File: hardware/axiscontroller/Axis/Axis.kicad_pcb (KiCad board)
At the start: 4 copper layers, 90 x 55 mm, 63 parts, among them J1 RS485, J10 Fan, J2 Motor, J3 Limits, J4 RS485, J5 Console, J6 Temp A, J7 Temp B, J8 Brake, J9 Power, Q4 IRLR8726TRPBF, Q5 IRLR8726TRPBF, SW1 SW_DIP_x04, U4 TLP291, U5 TLP291, U6 TLP291, U7 MAX485CPA, U8 74AHCT125

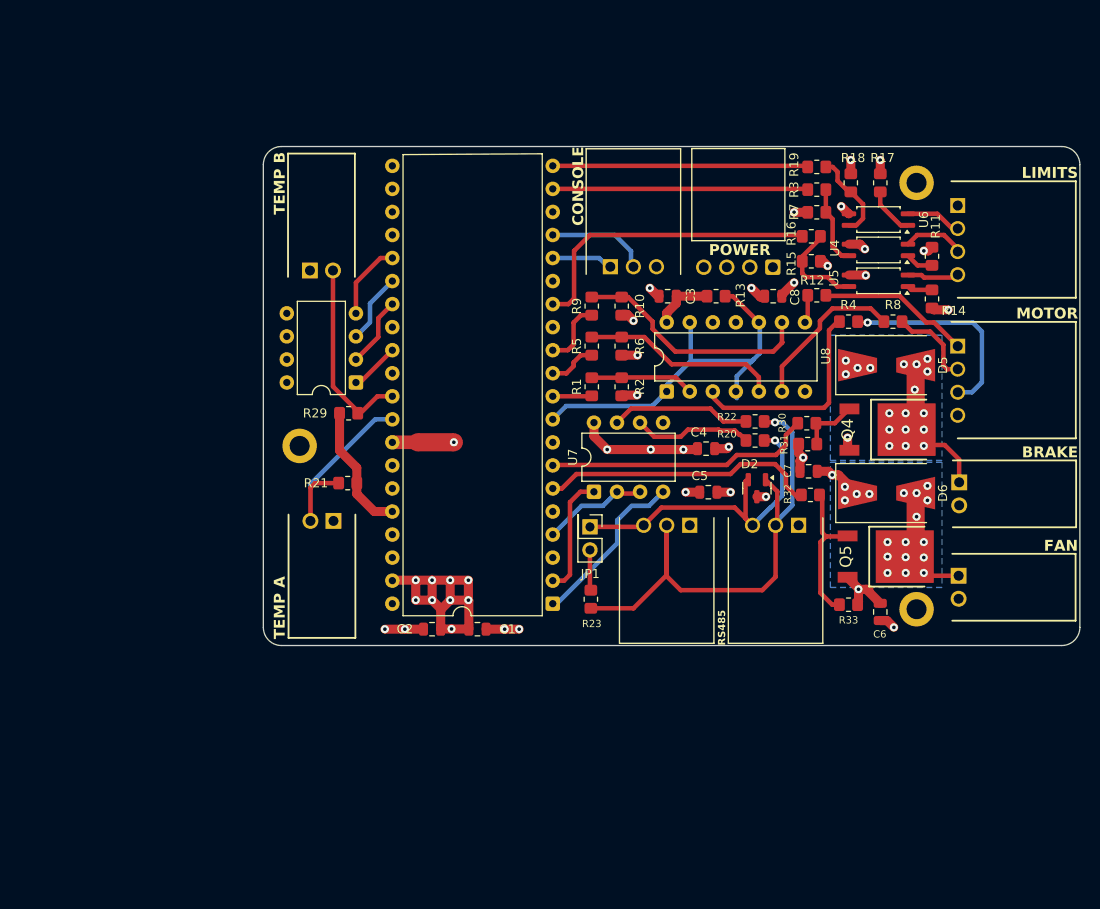
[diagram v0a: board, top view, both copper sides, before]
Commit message: The second revision of the robot axis controller.
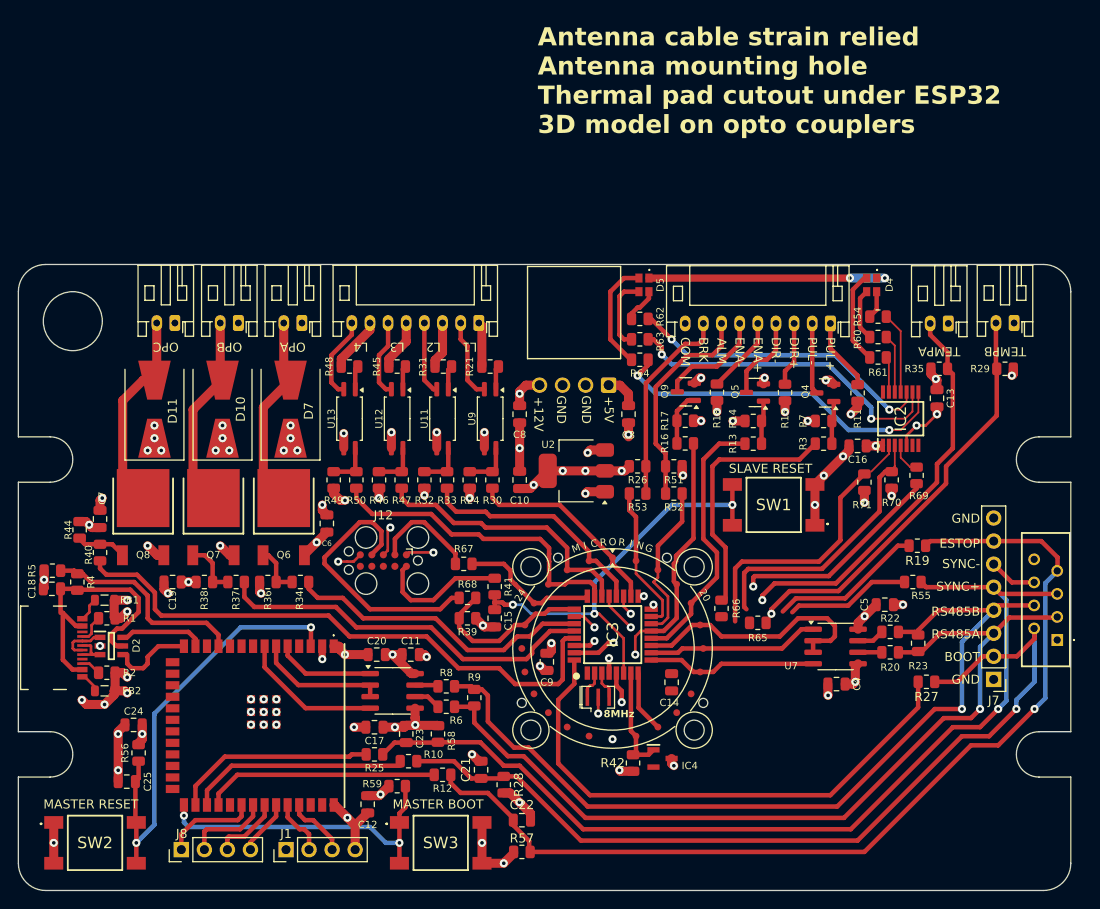
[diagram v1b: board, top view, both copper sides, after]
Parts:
- removed A1: RaspberryPi_Pico_W, AJS_Roberta:PI_PICO2_SOCKET
- removed C1: 100nF, Capacitor_SMD:C_0805_2012Metric
- removed C2: 47uF, Capacitor_SMD:C_0805_2012Metric
- removed D6: Schottky, Diode_SMD:D_SMB-SMC_Universal_Handsoldering
- removed H2, H3: MountingHole_Pad, MountingHole:MountingHole_2.2mm_M2_DIN965_Pad
- removed J10: Fan, AJS_Roberta:MOLEX_SL_70553_0001
- removed J9: Power, AJS_Roberta:MOLEX-171857-0001
- removed JP1: Termination, Connector_PinHeader_2.54mm:PinHeader_2x01_P2.54mm_Vertical
- removed NT1: NetTie_2, NetTie:NetTie-2_SMD_Pad2.0mm
- removed U4, U5, U6: TLP291, Package_SO:SOIC-4_4.55x2.6mm_P1.27mm
- removed U8: 74AHCT125, Package_DIP:DIP-14_W7.62mm
- added C10: 10uF, Capacitor_SMD:C_0805_2012Metric, F.Cu at (210.2, 103.8)
- added C11: 47uF, Capacitor_SMD:C_0805_2012Metric, F.Cu at (198.2, 123.0)
- added C12: 22uF, Capacitor_SMD:C_0805_2012Metric, F.Cu at (193.5, 139.5)
- added C13: 47uF, Capacitor_SMD:C_0805_2012Metric, F.Cu at (256.2, 94.8)
- added C14: 4.7uF, Capacitor_SMD:C_0805_2012Metric, F.Cu at (227.0, 126.0)
- added C15: 100nF, Capacitor_SMD:C_0805_2012Metric, F.Cu at (207.5, 119.0)
- added C16: 100nF, Capacitor_SMD:C_0805_2012Metric, F.Cu at (247.5, 100.0)
- added C17: 100nF, Capacitor_SMD:C_0805_2012Metric, F.Cu at (194.2, 131.0)
- added C18: 100nF, Capacitor_SMD:C_0805_2012Metric, F.Cu at (158.7, 115.8)
- added C19: 100nF, Capacitor_SMD:C_0805_2012Metric, F.Cu at (172.0, 115.0)
- added C20: 100nF, Capacitor_SMD:C_0805_2012Metric, F.Cu at (194.5, 123.0)
- added C21: 22nF, Capacitor_SMD:C_0805_2012Metric, F.Cu at (206.0, 135.7)
- added C22: 22nF, Capacitor_SMD:C_0805_2012Metric, F.Cu at (210.5, 141.2)
- added C23: 22nF, Capacitor_SMD:C_0805_2012Metric, F.Cu at (197.8, 131.8)
- added C24: 22uF, Capacitor_SMD:C_0805_2012Metric, F.Cu at (167.7, 130.8)
- added C25: 1uF, Capacitor_SMD:C_0805_2012Metric, F.Cu at (166.9, 137.0)
- added C9: 100nF, Capacitor_SMD:C_0805_2012Metric, F.Cu at (213.2, 123.8)
- added D10: Schottky, Diode_SMD:D_SMB-SMC_Universal_Handsoldering, F.Cu at (177.5, 96.0)
- added D11: Schottky, Diode_SMD:D_SMB-SMC_Universal_Handsoldering, F.Cu at (170.0, 96.0)
- added D4: CLMUD_FKC, AJS_Cree:CLMVC-FKC-CG1J1561BB7D3S3, F.Cu at (249.1, 82.2)
- added D7: Schottky, Diode_SMD:D_SMB-SMC_Universal_Handsoldering, F.Cu at (185.0, 96.0)
- added FB1: FerriteBead_Small, Inductor_SMD:L_0805_2012Metric, F.Cu at (164.5, 117.0)
- added FB2: FerriteBead_Small, Inductor_SMD:L_0805_2012Metric, F.Cu at (164.5, 127.0)
- added IC1: ESP32-S3-WROOM-1U-N16R8, AJS_Espressif:ESP32-S-3WROOM-1U-N16R8, F.Cu at (181.3, 130.8)
- added IC2: TCA6507PWR, AJS_TexasInstruments:TCA6507PWR, F.Cu at (252.2, 97.0)
- added IC3: STM32G071KBT3TR, AJS_STMicro:STM32G071KBT3TR, F.Cu at (220.5, 120.8)
- added IC4: AT21CS01-STUM10-T, AJS_STMicro:AT21CS01-STUM10-T, F.Cu at (226.0, 134.4)
- added J12: TC2050, Connector:Tag-Connect_TC2050-IDC-FP_2x05_P1.27mm_Vertical, F.Cu at (195.2, 112.6)
- added J17: JST PH, Connector_JST:JST_PH_S2B-PH-K_1x02_P2.00mm_Horizontal, F.Cu at (179.2, 86.5)
- added J18: JST PH, Connector_JST:JST_PH_S8B-PH-K_1x08_P2.00mm_Horizontal, F.Cu at (205.8, 86.5)
- added J19: JST PH, Connector_JST:JST_PH_S2B-PH-K_1x02_P2.00mm_Horizontal, F.Cu at (186.2, 86.5)
- added J20: JST PH, Connector_JST:JST_PH_S2B-PH-K_1x02_P2.00mm_Horizontal, F.Cu at (172.2, 86.5)
- added J21: JST PH, Connector_JST:JST_PH_S2B-PH-K_1x02_P2.00mm_Horizontal, F.Cu at (257.5, 86.5)
- added J22: JST PH, Connector_JST:JST_PH_S2B-PH-K_1x02_P2.00mm_Horizontal, F.Cu at (264.8, 86.5)
- added Q6: IRLR8726TRPBF, AJS_Roberta:IRLR8726TRPBF, F.Cu at (184.2, 107.8)
- added Q7: IRLR8726TRPBF, AJS_Roberta:IRLR8726TRPBF, F.Cu at (176.5, 107.8)
- added Q8: IRLR8726TRPBF, AJS_Roberta:IRLR8726TRPBF, F.Cu at (168.8, 107.8)
- added Q9: 2N7002, Package_TO_SOT_SMD:SOT-23, F.Cu at (228.6, 94.0)
- added R24: 4700, Resistor_SMD:R_0805_2012Metric, F.Cu at (204.8, 103.8)
- added R25: 33, Resistor_SMD:R_0805_2012Metric, F.Cu at (194.2, 134.0)
- added R26: 100K, Resistor_SMD:R_0805_2012Metric, F.Cu at (223.2, 102.2)
- added R27: 100, Resistor_SMD:R_0805_2012Metric, F.Cu at (255.1, 126.0)
- added R28: 4K7, Resistor_SMD:R_0805_2012Metric, F.Cu at (208.5, 137.3)
- added R34: 100, Resistor_SMD:R_0805_2012Metric, F.Cu at (186.1, 115.0)
- added R35: 10000, Resistor_SMD:R_0805_2012Metric, F.Cu at (256.5, 91.5)
- added R36: 10000, Resistor_SMD:R_0805_2012Metric, F.Cu at (182.5, 115.0)
- added R37: 100, Resistor_SMD:R_0805_2012Metric, F.Cu at (179.0, 115.0)
- added R38: 10000, Resistor_SMD:R_0805_2012Metric, F.Cu at (175.5, 115.0)
- added R39: 100K, Resistor_SMD:R_0805_2012Metric, F.Cu at (204.5, 119.0)
- added R40: 100, Resistor_SMD:R_0805_2012Metric, F.Cu at (164.0, 111.8)
- added R41: 100, Resistor_SMD:R_0805_2012Metric, F.Cu at (207.5, 115.5)
- added R42: 1K0, Resistor_SMD:R_0805_2012Metric, F.Cu at (222.8, 134.9)
- added R44: 10000, Resistor_SMD:R_0805_2012Metric, F.Cu at (161.8, 109.2)
- added R45: 1000, Resistor_SMD:R_0805_2012Metric, F.Cu at (196.8, 91.2)
- added R46: 4700, Resistor_SMD:R_0805_2012Metric, F.Cu at (194.8, 103.8)
- added R47: 100, Resistor_SMD:R_0805_2012Metric, F.Cu at (197.2, 103.8)
- added R48: 1000, Resistor_SMD:R_0805_2012Metric, F.Cu at (191.5, 91.2)
- added R49: 4700, Resistor_SMD:R_0805_2012Metric, F.Cu at (189.8, 103.8)
- added R50: 100, Resistor_SMD:R_0805_2012Metric, F.Cu at (192.2, 103.8)
- added R51: 100K, Resistor_SMD:R_0805_2012Metric, F.Cu at (227.2, 102.2)
- added R52: 100, Resistor_SMD:R_0805_2012Metric, F.Cu at (227.2, 105.2)
- added R53: 100, Resistor_SMD:R_0805_2012Metric, F.Cu at (223.2, 105.2)
- added R54: 330, Resistor_SMD:R_0805_2012Metric, F.Cu at (249.8, 85.8)
- added R55: 100, Resistor_SMD:R_0805_2012Metric, F.Cu at (253.6, 115.0)
- added R56: R_10K, Resistor_SMD:R_0805_2012Metric, F.Cu at (168.2, 133.8)
- added R57: 4K7, Resistor_SMD:R_0805_2012Metric, F.Cu at (210.5, 144.8)
- added R58: 4K7, Resistor_SMD:R_0805_2012Metric, F.Cu at (201.2, 131.8)
- added R59: R_10K, Resistor_SMD:R_0805_2012Metric, F.Cu at (196.8, 137.5)
- added R60: 330, Resistor_SMD:R_0805_2012Metric, F.Cu at (249.8, 88.0)
- added R61: 330, Resistor_SMD:R_0805_2012Metric, F.Cu at (249.8, 90.2)
- added R62: 330, Resistor_SMD:R_0805_2012Metric, F.Cu at (223.5, 86.0)
- added R63: 330, Resistor_SMD:R_0805_2012Metric, F.Cu at (223.5, 88.2)
- added R64: 330, Resistor_SMD:R_0805_2012Metric, F.Cu at (223.5, 90.5)
- added R65: 33, Resistor_SMD:R_0805_2012Metric, F.Cu at (236.5, 119.5)
- added R66: 33, Resistor_SMD:R_0805_2012Metric, F.Cu at (232.5, 117.9)
- added R67: 33, Resistor_SMD:R_0805_2012Metric, F.Cu at (204.1, 113.0)
- added R68: 33, Resistor_SMD:R_0805_2012Metric, F.Cu at (204.5, 116.8)
- added R69: 33, Resistor_SMD:R_0805_2012Metric, F.Cu at (254.0, 103.2)
- added R70: 4K7, Resistor_SMD:R_0805_2012Metric, F.Cu at (251.2, 103.8)
- added R71: 4K7, Resistor_SMD:R_0805_2012Metric, F.Cu at (248.2, 104.0)
- added SW2: SW_Tactile_6mm, AJS_SameSky:Tactile_6mm_6mm_4.5mm, F.Cu at (163.4, 143.8)
- added SW3: SW_Tactile_6mm, AJS_SameSky:Tactile_6mm_6mm_4.5mm, F.Cu at (201.6, 143.8)
- added U11: TLP291, Package_SO:SOIC-4_4.55x2.6mm_P1.27mm, F.Cu at (201.8, 97.0)
- added U12: TLP291, Package_SO:SOIC-4_4.55x2.6mm_P1.27mm, F.Cu at (196.8, 97.0)
- added U13: TLP291, Package_SO:SOIC-4_4.55x2.6mm_P1.27mm, F.Cu at (191.5, 97.0)
- added U14: MAX485CPA, Package_SO:SOIC-8_3.9x4.9mm_P1.27mm, F.Cu at (196.2, 127.0)
- added U2: AMS1117-3.3, Package_TO_SOT_SMD:SOT-223-3_TabPin2, F.Cu at (216.5, 102.8)
- added U9: TLP291, Package_SO:SOIC-4_4.55x2.6mm_P1.27mm, F.Cu at (207.0, 97.0)
- added Y4: 8MHz, Crystal:Resonator_SMD_Murata_CSTxExxV-3Pin_3.0x1.1mm, F.Cu at (218.9, 127.7)
- C3: value 100nF -> 10uF
- D2: value SM712_SOT23 -> USBLC6-2SC6Y; footprint Package_TO_SOT_SMD:SOT-23 -> AJS_STMicro:USBLC6-2SC6Y
- D5: value Schottky -> CLMUD_FKC; footprint Diode_SMD:D_SMB-SMC_Universal_Handsoldering -> AJS_Cree:CLMVC-FKC-CG1J1561BB7D3S3
- H1: value MountingHole_Pad -> MountingHole; footprint MountingHole:MountingHole_2.2mm_M2_DIN965_Pad -> MountingHole:MountingHole_6.5mm
- J1: value RS485 -> Conn_01x04_Pin; footprint AJS_Roberta:MOLEX_SL_70553_0002 -> Connector_PinHeader_2.54mm:PinHeader_1x04_P2.54mm_Vertical
- J2: value Motor -> CL57_Driver; footprint AJS_Roberta:MOLEX_SL_70553_0003 -> Connector_JST:JST_PH_S9B-PH-K_1x09_P2.00mm_Horizontal
- J3: value Limits -> ~; footprint AJS_Roberta:MOLEX_SL_70553_0003 -> AJS_Molex:KK254-171857-0004
- J4: value RS485 -> Conn_02x12_Counter_Clockwise; footprint AJS_Roberta:MOLEX_SL_70553_0002 -> AJS_UProbe:MicroRing24x20
- J5: value Console -> USBC-217179-0001; footprint AJS_Roberta:MOLEX_SL_70553_0002 -> AJS_Molex:USBC-217179-0001
- J6: value Temp A -> TE MicroMatch; footprint AJS_Roberta:MOLEX_SL_70553_0001 -> AJS_TEConnectivity:MicroMatch_Locking_3380708
- J7: value Temp B -> ~; footprint AJS_Roberta:MOLEX_SL_70553_0001 -> Connector_PinHeader_2.54mm:PinHeader_1x08_P2.54mm_Vertical
- J8: value Brake -> Conn_01x04_Pin; footprint AJS_Roberta:MOLEX_SL_70553_0001 -> Connector_PinHeader_2.54mm:PinHeader_1x04_P2.54mm_Vertical
- Q4, Q5: value IRLR8726TRPBF -> 2N7002; footprint AJS_Roberta:IRLR8726TRPBF -> Package_TO_SOT_SMD:SOT-23
- R1: value 100 -> 5K1; footprint Resistor_SMD:R_0805_2012Metric_Pad1.20x1.40mm_HandSolder -> Resistor_SMD:R_0805_2012Metric
- R10: value 10000 -> 33; footprint Resistor_SMD:R_0805_2012Metric_Pad1.20x1.40mm_HandSolder -> Resistor_SMD:R_0805_2012Metric
- R11: value 1000 -> 0; footprint Resistor_SMD:R_0805_2012Metric_Pad1.20x1.40mm_HandSolder -> Resistor_SMD:R_0805_2012Metric
- R12: value 470 -> 33; footprint Resistor_SMD:R_0805_2012Metric_Pad1.20x1.40mm_HandSolder -> Resistor_SMD:R_0805_2012Metric
- R13, R33: value 10000 -> 100; footprint Resistor_SMD:R_0805_2012Metric_Pad1.20x1.40mm_HandSolder -> Resistor_SMD:R_0805_2012Metric
- R14, R17: value 1000 -> 100k; footprint Resistor_SMD:R_0805_2012Metric_Pad1.20x1.40mm_HandSolder -> Resistor_SMD:R_0805_2012Metric
- R15, R18: value 4700 -> 0; footprint Resistor_SMD:R_0805_2012Metric_Pad1.20x1.40mm_HandSolder -> Resistor_SMD:R_0805_2012Metric
- R16, R19, R20, R22, R23, R29, R3, R30: footprint Resistor_SMD:R_0805_2012Metric_Pad1.20x1.40mm_HandSolder -> Resistor_SMD:R_0805_2012Metric
- R2: value 10000 -> 5K1; footprint Resistor_SMD:R_0805_2012Metric_Pad1.20x1.40mm_HandSolder -> Resistor_SMD:R_0805_2012Metric
- R21, R31: value 10000 -> 1000; footprint Resistor_SMD:R_0805_2012Metric_Pad1.20x1.40mm_HandSolder -> Resistor_SMD:R_0805_2012Metric
- R32: value 100 -> 4700; footprint Resistor_SMD:R_0805_2012Metric_Pad1.20x1.40mm_HandSolder -> Resistor_SMD:R_0805_2012Metric
- R4: value 470 -> 4K7; footprint Resistor_SMD:R_0805_2012Metric_Pad1.20x1.40mm_HandSolder -> Resistor_SMD:R_0805_2012Metric
- R5: value 100 -> 100K; footprint Resistor_SMD:R_0805_2012Metric_Pad1.20x1.40mm_HandSolder -> Resistor_SMD:R_0805_2012Metric
- R6: value 10000 -> 47; footprint Resistor_SMD:R_0805_2012Metric_Pad1.20x1.40mm_HandSolder -> Resistor_SMD:R_0805_2012Metric
- R7: value 4700 -> 100k; footprint Resistor_SMD:R_0805_2012Metric_Pad1.20x1.40mm_HandSolder -> Resistor_SMD:R_0805_2012Metric
- R8: value 470 -> 47; footprint Resistor_SMD:R_0805_2012Metric_Pad1.20x1.40mm_HandSolder -> Resistor_SMD:R_0805_2012Metric
- R9: value 100 -> 120; footprint Resistor_SMD:R_0805_2012Metric_Pad1.20x1.40mm_HandSolder -> Resistor_SMD:R_0805_2012Metric
- SW1: value SW_DIP_x04 -> SW_Tactile_6mm; footprint Package_DIP:DIP-8_W7.62mm -> AJS_SameSky:Tactile_6mm_6mm_4.5mm
- U7: footprint Package_DIP:DIP-8_W7.62mm -> Package_SO:SOIC-8_3.9x4.9mm_P1.27mm
- moved J8 104.9 mm to (173.0, 144.5), turned to 90 degrees
- moved H1 94.2 mm to (161.0, 86.2)
- moved J7 92.5 mm to (262.5, 125.7), turned to 180 degrees
- moved R4 89.7 mm to (161.5, 115.0), turned to 90 degrees
- moved J5 83.9 mm to (158.8, 122.2), turned to -90 degrees
- moved J6 82.4 mm to (269.5, 121.4), turned to 90 degrees
- moved C7 78.3 mm to (164.0, 108.0), turned to -90 degrees
- moved D2 73.2 mm to (165.2, 122.0), turned to 0 degrees
- moved R29 72.5 mm to (263.8, 91.5), turned to 0 degrees
- moved R12 67.0 mm to (201.8, 136.2)
- moved R2 64.9 mm to (164.8, 125.0), turned to 0 degrees
- moved R5 64.4 mm to (158.8, 113.8), turned to 180 degrees
- moved R8 63.6 mm to (202.2, 126.5), turned to 180 degrees
- moved C6 61.8 mm to (189.0, 108.5), turned to -90 degrees
- moved R1 59.2 mm to (164.8, 119.0), turned to 0 degrees
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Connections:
- C4 pad 1: +5V -> +3V3
- C5 pad 1: +5V -> +3V3
- D2 pad 1: Net-(D2-A1) -> Net-(D2-I/O1_1)
- D2 pad 2: Net-(D2-A2) -> GND
- D2 pad 3: GND -> Net-(D2-I/O2_1)
- D5 pad 1: +12V -> +3V3
- D5 pad 2: Net-(D5-A) -> Net-(D5-RK)
- J1 pad 1: GND -> +3V3
- J1 pad 2: Net-(D2-A1) -> /Master/CONSOLE_RX
- J1 pad 3: Net-(D2-A2) -> /Master/CONSOLE_TX
- J2 pad 1: /ENA -> /PUL+
- J2 pad 2: /DIR -> /PUL-
- J2 pad 3: /PUL -> /DIR+
- J2 pad 4: GND -> /DIR-
- J3 pad 1: GND -> +5V
- J3 pad 2: /HOME -> GND
- J3 pad 3: /LIMIT_A -> GND
- J3 pad 4: /LIMIT_B -> +12V
- J4 pad 1: GND -> /LIMIT_A
- J4 pad 2: Net-(D2-A1) -> /LIMIT_B
- J4 pad 3: Net-(D2-A2) -> /LIMIT_C
- J6 pad 2: Net-(A1-GPIO27_ADC1) -> /BOOT
- J7 pad 2: Net-(A1-GPIO26_ADC0) -> /BOOT
- J8 pad 1: Net-(D5-A) -> /Master/TCK
- J8 pad 2: +12V -> /Master/TDO
- Q4 pad 2: Net-(D5-A) -> GND
- Q4 pad 3: GND -> /PUL-
- Q5 pad 2: Net-(D6-A) -> GND
- Q5 pad 3: GND -> /DIR-
- R1 pad 1: /MCU_PUL -> Net-(J5-CC1)
- R1 pad 2: Net-(R1-Pad2) -> GND
- R10 pad 1: GND -> /Master/MCU_BOOT
- R10 pad 2: Net-(R10-Pad2) -> /BOOT
- R11 pad 1: +12V -> +5V
- R11 pad 2: Net-(R11-Pad2) -> /PUL+
- R12 pad 1: Net-(R12-Pad1) -> /Master/MCU_ESTOP
- R12 pad 2: /ENA -> /ESTOP
- R13 pad 1: /MOTOR_OE -> /MCU_DIR
- R13 pad 2: +5V -> Net-(Q5-G)
- R14 pad 1: +12V -> GND
- R14 pad 2: Net-(R14-Pad2) -> Net-(Q5-G)
- R15 pad 1: Net-(R15-Pad1) -> +5V
- R15 pad 2: +5V -> /DIR+
- R16 pad 1: Net-(R15-Pad1) -> /MCU_ENA
- R16 pad 2: /MCU_LIMIT_B -> Net-(Q9-G)
- R17 pad 1: +12V -> GND
- R17 pad 2: Net-(R17-Pad2) -> Net-(Q9-G)
- R18 pad 1: Net-(R18-Pad1) -> +5V
- R18 pad 2: +5V -> /ENA+
- R19 pad 1: Net-(R18-Pad1) -> /ESTOP
- R19 pad 2: /MCU_HOME -> /MicroController/ESTOP
- R2 pad 1: GND -> Net-(J5-CC2)
- R2 pad 2: Net-(R1-Pad2) -> GND
- R20 pad 1: Net-(D2-A2) -> /RS485_A
- R21 pad 1: Net-(A1-GPIO27_ADC1) -> +12V
- R21 pad 2: +3V3 -> Net-(R21-Pad2)
- R22 pad 1: Net-(D2-A1) -> /RS485_B
- R23 pad 1: Net-(JP1-B) -> /RS485_A
- R23 pad 2: Net-(D2-A1) -> /RS485_B
- R29 pad 1: Net-(A1-GPIO26_ADC0) -> /MicroController/TEMP_B
- R3 pad 1: Net-(R3-Pad1) -> /MCU_PUL
- R3 pad 2: /MCU_LIMIT_A -> Net-(Q4-G)
- R30 pad 1: Net-(Q4-G) -> Net-(R24-Pad1)
- R30 pad 2: /MCU_BRAKE -> /LIMIT_A
- R31 pad 1: Net-(Q4-G) -> +12V
- R31 pad 2: GND -> Net-(R31-Pad2)
- R32 pad 1: Net-(Q5-G) -> Net-(R32-Pad1)
- R32 pad 2: /MCU_FAN -> +3V3
- R33 pad 1: Net-(Q5-G) -> Net-(R32-Pad1)
- R33 pad 2: GND -> /LIMIT_B
- R4 pad 1: Net-(R4-Pad1) -> Net-(D2-VBUS)
- R4 pad 2: /PUL -> /Master/USB_SENSE
- R5 pad 1: /MCU_DIR -> /Master/USB_SENSE
- R5 pad 2: Net-(R5-Pad2) -> GND
- R6 pad 1: GND -> /RS485_A
- R6 pad 2: Net-(R5-Pad2) -> Net-(U14-A)
- R7 pad 1: Net-(R3-Pad1) -> GND
- R7 pad 2: +5V -> Net-(Q4-G)
- R8 pad 1: Net-(R8-Pad1) -> /RS485_B
- R8 pad 2: /DIR -> Net-(U14-B)
- R9 pad 1: /MCU_ENA -> /RS485_A
- R9 pad 2: Net-(R10-Pad2) -> /RS485_B
- SW1 pad 1: /ADDR0 -> GND
- SW1 pad 2: /ADDR1 -> /MicroController/NRST
- U7 pad 1: /RS485_RX -> /MicroController/RS485_RX
- U7 pad 2: /RS485_DIR -> /MicroController/RS485_DIR
- U7 pad 3: /RS485_DIR -> /MicroController/RS485_DIR
- U7 pad 4: /RS485_TX -> /MicroController/RS485_TX
- U7 pad 8: +5V -> +3V3
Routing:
- net /ESTOP: track 0.00 -> 109.3 mm, vias 0 -> 1
- net /SYNC: track 0.00 -> 107.8 mm, vias 0 -> 1
- net /BOOT: track 0.00 -> 99.7 mm, vias 0 -> 1
- net GND: track 37.1 -> 135.6 mm, vias 19 -> 63
- net /RS485_A: track 0.00 -> 97.2 mm, vias 0 -> 1
- net /RS485_B: track 0.00 -> 96.6 mm, vias 0 -> 1
- net +3V3: track 14.4 -> 80.1 mm, vias 0 -> 28
- net /OP_SPARE: track 0.00 -> 64.0 mm
- net Net-(D2-A1): track 60.2 -> 0.00 mm, vias 1 -> 0
- net /MicroController/BOOT: track 0.00 -> 60.0 mm
- net Net-(IC1-EN): track 0.00 -> 49.8 mm, vias 0 -> 2
- net /MicroController/NRST: track 0.00 -> 48.0 mm, vias 0 -> 3
- net +5V: track 57.9 -> 10.1 mm, vias 16 -> 4
- net /MicroController/TEMP_B: track 0.00 -> 46.1 mm, vias 0 -> 2
- net /MicroController/TEMP_A: track 0.00 -> 44.8 mm, vias 0 -> 2
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- added copper zone on In2.Cu, net +12V
- added copper zone on In2.Cu, net +3V3
- added copper zone on In2.Cu, net +5V
- added copper zone on In1.Cu, net GND
- removed copper zone on In1.Cu, net +12V
- removed copper zone on In1.Cu, net +5V
- removed copper zone on In2.Cu, net GND
- removed copper zone on B.Cu, net Net-(D5-A)
- removed copper zone on B.Cu, net Net-(D6-A)
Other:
- board size 90 x 55 mm -> 116 x 69 mm
- board text added: "8MHz"
- board text added: "ALM"
- board text added: "Antenna cable strain relied Antenna mounting hole Thermal pad cutout under ESP32 3D model on opto couplers"
- board text added: "BOOT"
- board text added: "BRK"
- board text added: "COM"
- board text added: "DIR+"
- board text added: "DIR-"
- board text added: "ENA+"
- board text added: "ENA-"
- board text added: "ESTOP"
- board text added: "L1"
- board text added: "L2"
- board text added: "L3"
- board text added: "L4"
- board text added: "MASTER BOOT"
- board text added: "MASTER RESET"
- board text added: "OPA"
- board text added: "OPB"
- board text added: "OPC"
- board text added: "PUL+"
- board text added: "PUL-"
- board text added: "RS485A"
- board text added: "RS485B"
- board text added: "SLAVE RESET"
- board text added: "SYNC+"
- board text added: "SYNC-"
- board text added: "TEMPA"
- board text added: "TEMPB"
- board text removed: "18mm"
- board text removed: "22mm"
- board text removed: "33mm"
- board text removed: "4mm"
- board text removed: "72mm"
- board text removed: "A"
- board text removed: "B"
- board text removed: "BRAKE"
- board text removed: "BRAKE+"
- board text removed: "BRAKE-"
- board text removed: "CONSOLE"
- board text removed: "DIR"
- board text removed: "ENA"
- board text removed: "FAN"
- board text removed: "FAN+"
- board text removed: "FAN-"
- board text removed: "HOME"
- board text removed: "LIMIT A"
- board text removed: "LIMIT B"
- board text removed: "LIMITS"
- board text removed: "M2"
- board text removed: "MOTOR"
- board text removed: "POWER"
- board text removed: "PUL"
- board text removed: "RS485"
- board text removed: "RX"
- board text removed: "Rev A, AJS Contract Design Ltd, 2025"
- board text removed: "SENSOR"
- board text removed: "Single Axis Controller"
- board text removed: "TEMP A"
- board text removed: "TEMP B"
- board text removed: "TX"
